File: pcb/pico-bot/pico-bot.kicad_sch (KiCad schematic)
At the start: 38 parts

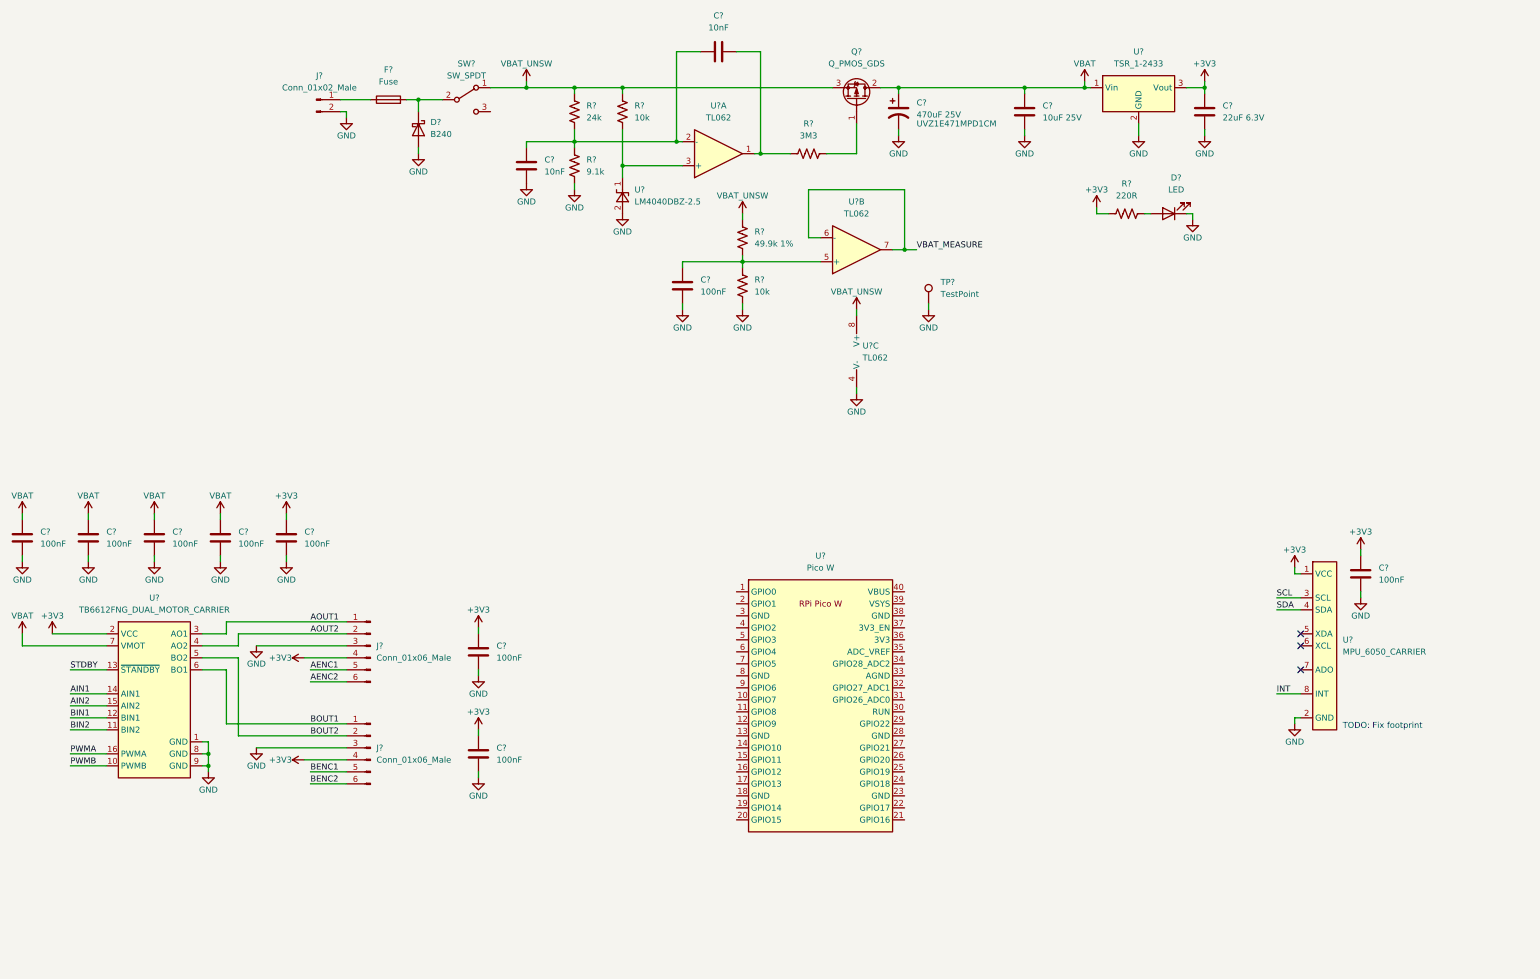
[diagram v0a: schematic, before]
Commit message: Progress commit
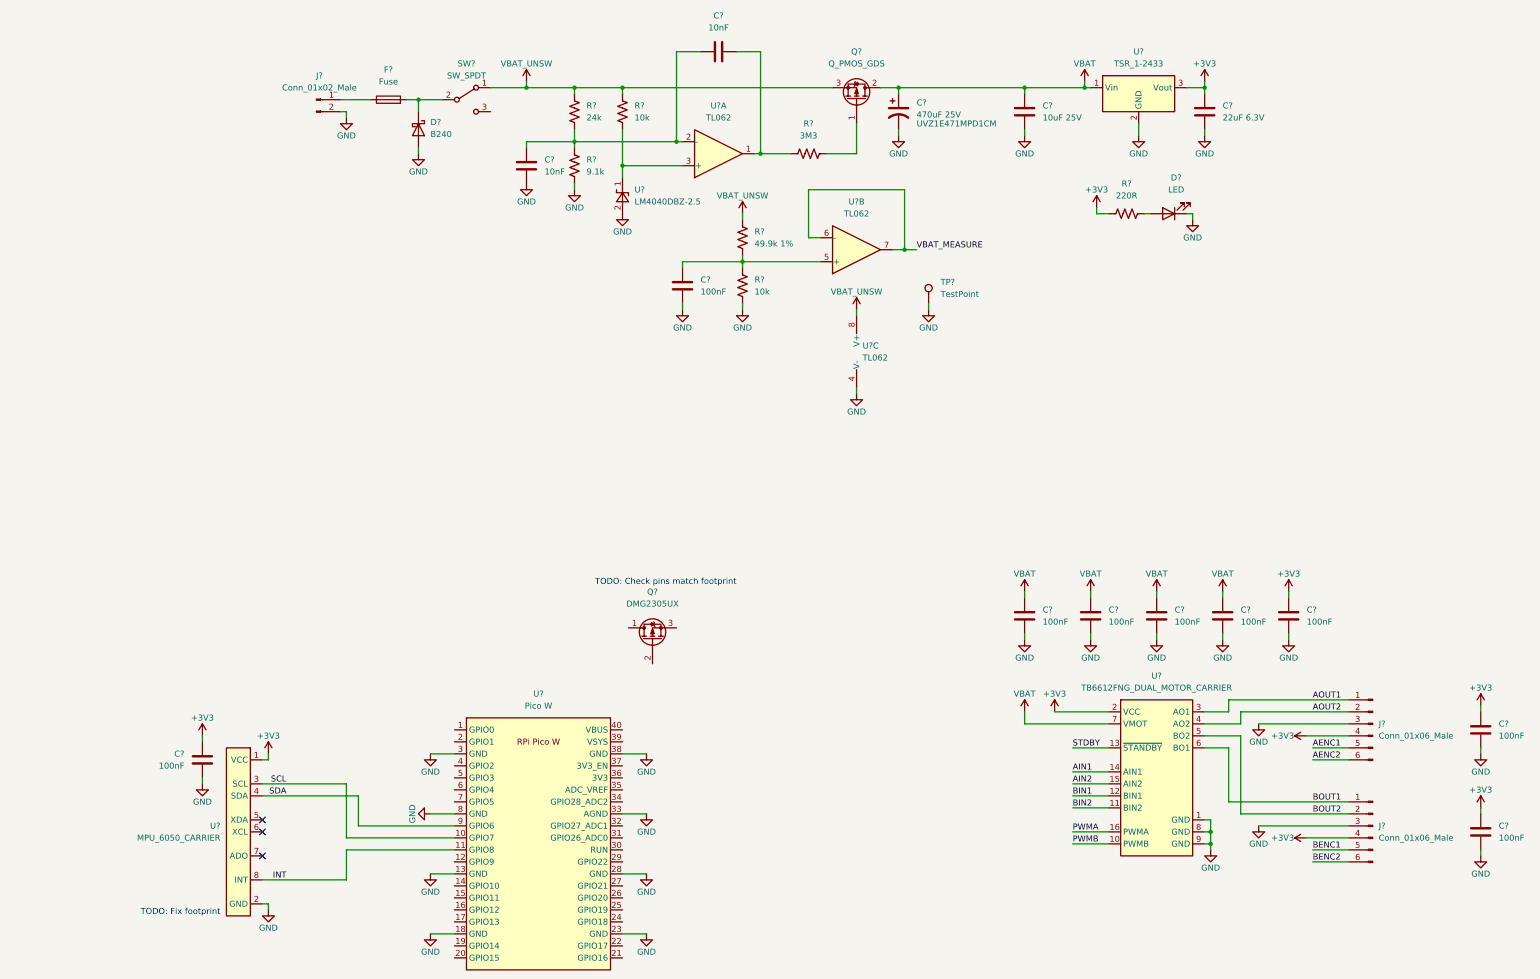
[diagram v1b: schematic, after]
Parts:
- added Q?: DMG2305UX, symbol Device:Q_PMOS_DGS
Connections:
- net GND: now also U?.13 (GND), U?.18 (GND), U?.23 (GND), U?.28 (GND), U?.3 (GND), U?.33 (AGND), U?.38 (GND), U?.8 (GND)
- net INT: now also U?.11 (GPIO8)
- net SCL: now also U?.10 (GPIO7)
- net SDA: now also U?.9 (GPIO6)
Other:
- note added: "TODO: Check pins match footprint"
- moved on the sheet: C?, J?, U?
